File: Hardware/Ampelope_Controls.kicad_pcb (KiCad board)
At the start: 2 copper layers, 60.5 x 110 mm, 36 parts, among them J1 Conn_01x12_Male, J10 Audio2_In, J11 Audio3_In, J12 Audio4_In, J13 Audio1_Out, J14 Audio2_Out, J15 Audio3_Out, J16 Audio4_Out, J17 Clock_In, J18 Env1_Out, J19 Env2_Out, J2 Conn_01x12_Male, J3 Conn_01x12_Male, J4 Conn_01x12_Male, J5 Gate1_In, J6 Gate2_In, J7 Gate3_In, J8 Gate4_In, J9 Audio1_In

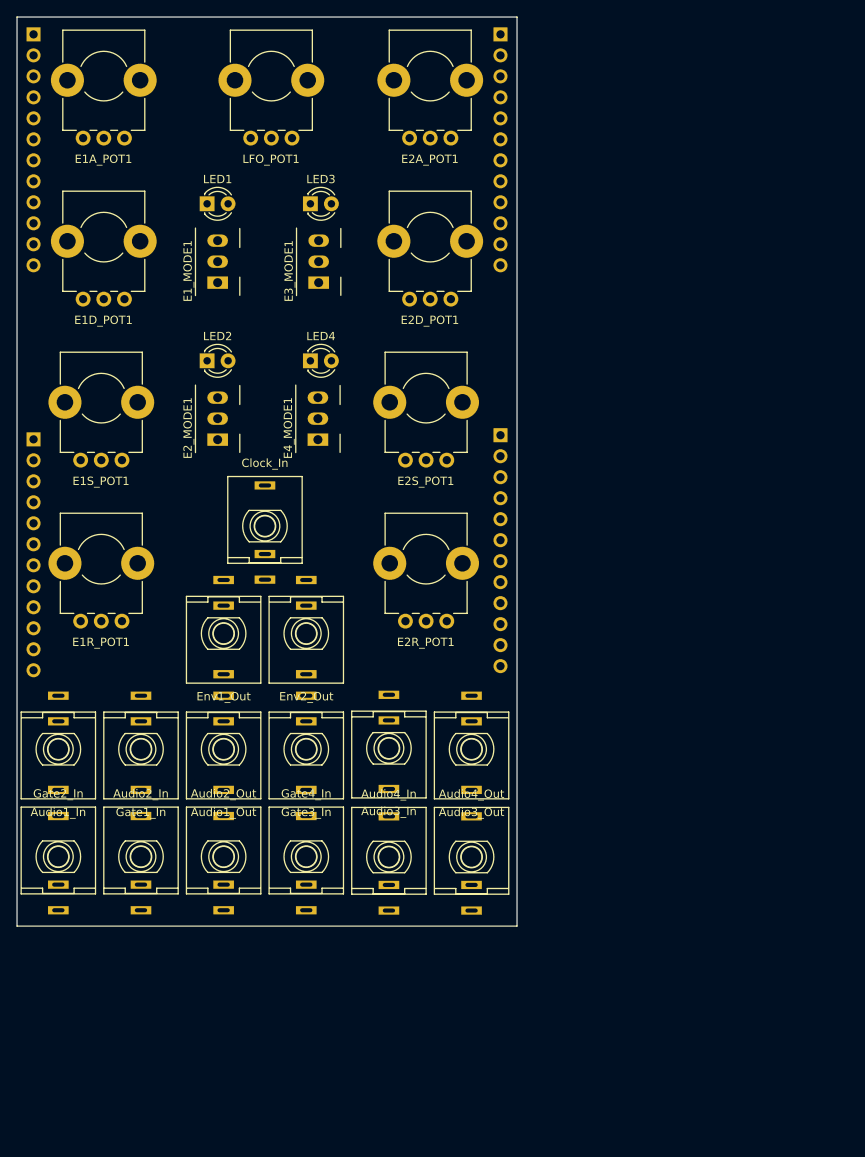
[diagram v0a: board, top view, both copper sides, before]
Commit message: Work on panel and control layout
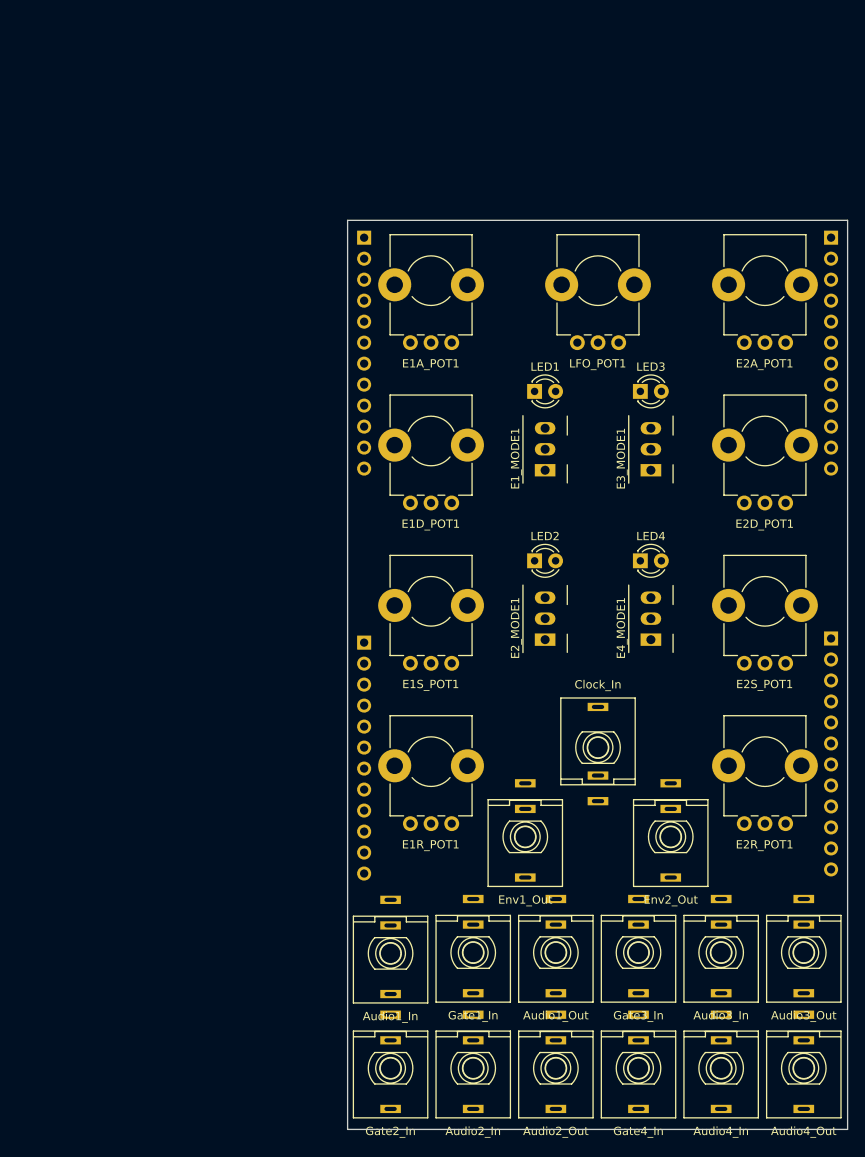
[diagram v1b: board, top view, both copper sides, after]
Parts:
- moved J19 50.5 mm to (139.1, 124.6)
- moved J17 48.4 mm to (130.3, 113.8)
- moved E2S_POT1 47.8 mm to (150.5, 96.1)
- moved E2R_POT1 47.8 mm to (150.5, 115.5)
- moved J10 47.7 mm to (115.2, 152.6), turned to 180 degrees
- moved J14 47.7 mm to (125.2, 152.6), turned to 180 degrees
- moved J6 47.7 mm to (105.2, 152.6), turned to 180 degrees
- moved J8 47.7 mm to (135.2, 152.6), turned to 180 degrees
- moved J12 47.6 mm to (145.2, 152.6), turned to 180 degrees
- moved J16 47.6 mm to (155.2, 152.6), turned to 180 degrees
- moved E2A_POT1 47.5 mm to (150.5, 57.3)
- moved E2D_POT1 47.4 mm to (150.5, 76.7)
- moved J11 47.2 mm to (145.2, 138.6)
- moved J9 47.2 mm to (105.2, 138.7)
- moved J13 47.1 mm to (125.2, 138.6)
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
